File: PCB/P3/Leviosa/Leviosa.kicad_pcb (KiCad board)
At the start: 2 copper layers, 78.2 x 75.4 mm, 55 parts, among them J1 Barrel_Jack, J2 2.54mm 1x03 Spare, Q1 NCE0110K

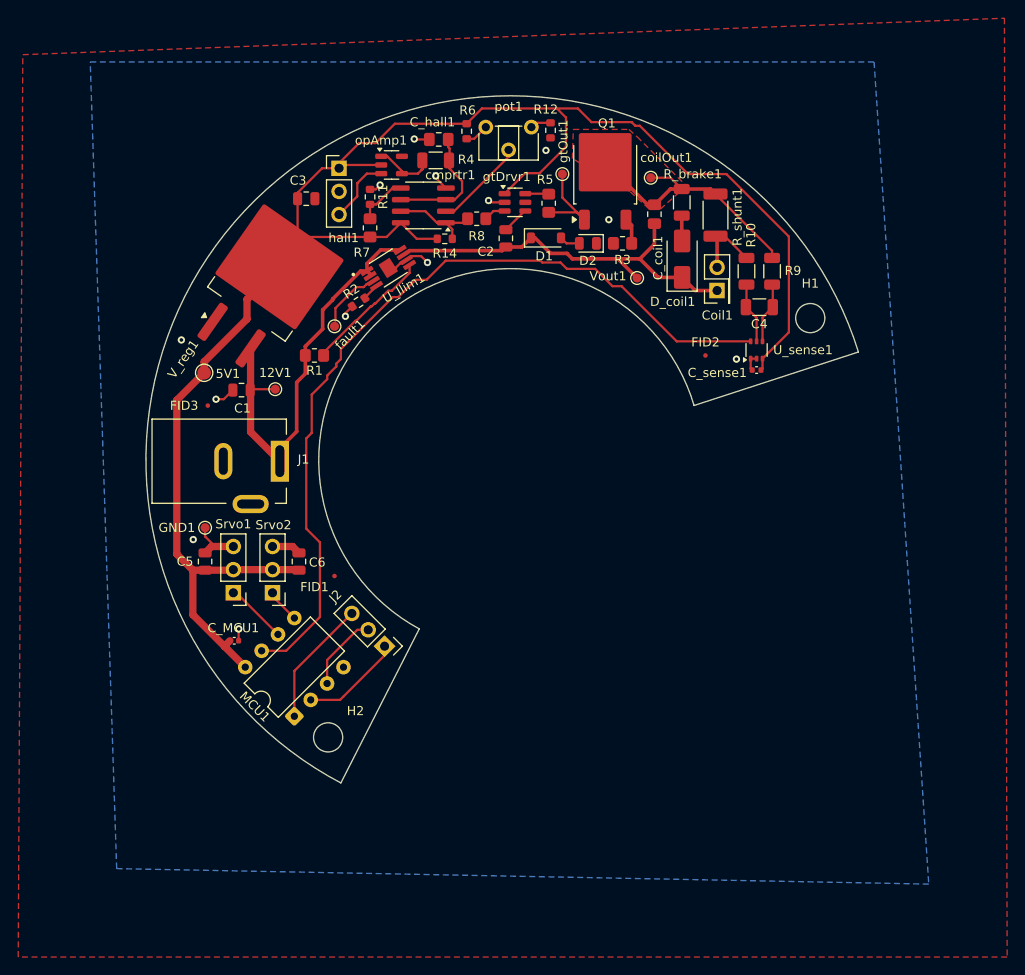
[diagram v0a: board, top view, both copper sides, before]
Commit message: Board revised
- Big change from the last so have a look over
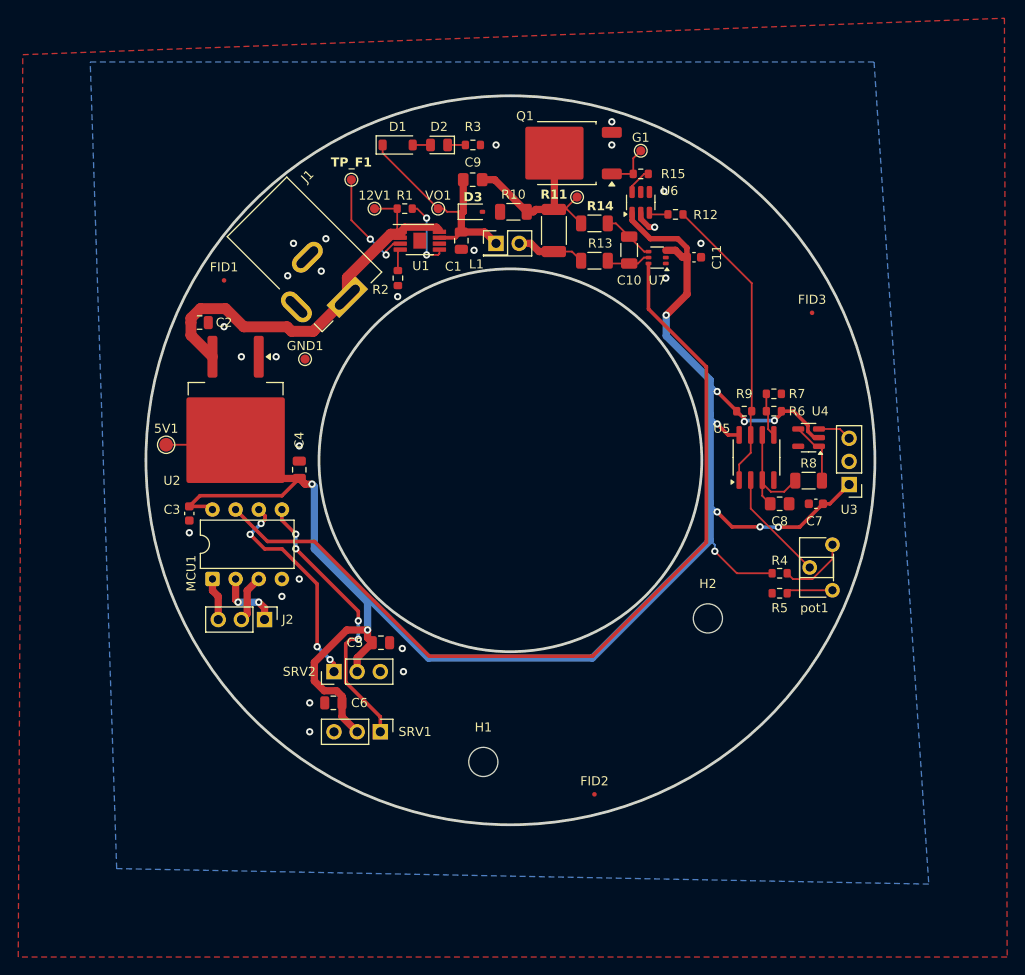
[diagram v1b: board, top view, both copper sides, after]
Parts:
- removed C_MCU1, C_sense1: 0.1µF, Capacitor_SMD:C_0402_1005Metric
- removed C_coil1: 20nF, Capacitor_SMD:C_0805_2012Metric_Pad1.18x1.45mm_HandSolder
- removed C_hall1: 4.7nF, Capacitor_SMD:C_0805_2012Metric_Pad1.18x1.45mm_HandSolder
- removed Coil1: 7.4mH, Connector_PinHeader_2.54mm:PinHeader_2x01_P2.54mm_Vertical
- removed D_coil1: SS34, Diode_SMD:D_SMA
- removed R_brake1: 8.2Ω, Resistor_SMD:R_1206_3216Metric
- removed R_shunt1: 50mΩ, Resistor_SMD:R_2010_5025Metric
- removed Srvo1, Srvo2: 2.54mm 1x03 Servo 1, Connector_PinHeader_2.54mm:PinHeader_1x03_P2.54mm_Vertical
- removed U_Ilim1: TPS1H200AQDGNRQ1, TPS1H200AQDGNRQ1:SOP65P490X110-9N
- removed U_sense1: INA199xxDCK (50V/V), Package_TO_SOT_SMD:SOT-363_SC-70-6
- removed V_reg1: MC7805BD2TR4G, Package_TO_SOT_SMD:TO-263-2
- removed Vout1: Vout, TestPoint:TestPoint_Pad_D1.0mm
- removed cmprtr1: LM393, Package_SO:SOIC-8_3.9x4.9mm_P1.27mm
- removed coilOut1: coil_out, TestPoint:TestPoint_Pad_D1.0mm
- removed fault1: Fault, TestPoint:TestPoint_Pad_D1.0mm
- removed gtDrvr1: MX27517, Package_TO_SOT_SMD:SOT-23-6
- removed gtOut1: set_point_trigger, TestPoint:TestPoint_Pad_D1.0mm
- removed hall1: SS495A, Connector_PinHeader_2.54mm:PinHeader_1x03_P2.54mm_Vertical
- removed opAmp1: MCP6001R, Package_TO_SOT_SMD:SOT-23-5
- added C10: 47μF, Capacitor_SMD:C_1206_3216Metric, F.Cu at (113.0, 76.9)
- added C11: 0.1µF, Capacitor_SMD:C_0603_1608Metric, F.Cu at (120.1, 77.7)
- added C7: 0.1uF, Capacitor_SMD:C_0603_1608Metric, F.Cu at (133.5, 104.8)
- added C8: 4.7nF, Capacitor_SMD:C_0805_2012Metric_Pad1.18x1.45mm_HandSolder, F.Cu at (129.5, 104.8)
- added C9: 20nF, Capacitor_SMD:C_0805_2012Metric_Pad1.18x1.45mm_HandSolder, F.Cu at (95.9, 69.2)
- added D3: SS34, Diode_SMD:D_SOD-323, F.Cu at (95.9, 72.7)
- added G1: set_point_trigger, TestPoint:TestPoint_Pad_D1.0mm, F.Cu at (114.3, 66.0)
- added L1: 7.4mH, Connector_PinHeader_2.54mm:PinHeader_2x01_P2.54mm_Vertical, F.Cu at (98.4, 76.2)
- added R13: 8.2Ω, Resistor_SMD:R_1206_3216Metric, F.Cu at (109.2, 78.1)
- added R15: 0Ω, Resistor_SMD:R_0603_1608Metric, F.Cu at (114.3, 68.6)
- added SRV1: 2.54mm 1x03 Servo 1, Connector_PinHeader_2.54mm:PinHeader_1x03_P2.54mm_Vertical, F.Cu at (85.7, 129.8)
- added SRV2: 2.54mm 1x03 Servo 1, Connector_PinHeader_2.54mm:PinHeader_1x03_P2.54mm_Vertical, F.Cu at (80.6, 123.2)
- added TP_COIL1: Coil Output, TestPoint:TestPoint_Pad_D1.0mm, F.Cu at (107.3, 71.1)
- added TP_F1: Fault, TestPoint:TestPoint_Pad_D1.0mm, F.Cu at (82.5, 69.2)
- added U1: TPS1H200AQDGNRQ1, TPS1H200AQDGNRQ1:SOP65P490X110-9N, F.Cu at (90.1, 75.9)
- added U2: MC7805BD2TR4G, Package_TO_SOT_SMD:TO-263-2, F.Cu at (69.8, 96.3)
- added U3: SS495A, Connector_PinHeader_2.54mm:PinHeader_1x03_P2.54mm_Vertical, F.Cu at (137.2, 102.7)
- added U4: MCP6001R, Package_TO_SOT_SMD:SOT-23-5, F.Cu at (132.7, 97.5)
- added U5: LM393, Package_SO:SOIC-8_3.9x4.9mm_P1.27mm, F.Cu at (127.0, 99.7)
- added U6: MX27517, Package_TO_SOT_SMD:SOT-23-6, F.Cu at (114.3, 71.7)
- added U7: INA199xxDCK (50V/V), Package_TO_SOT_SMD:SOT-363_SC-70-6, F.Cu at (116.1, 77.8)
- added VO1: Vout, TestPoint:TestPoint_Pad_D1.0mm, F.Cu at (92.1, 72.4)
- C1: value 0.33µF -> 22µF
- C2: value 22µF -> 0.33µF
- C3: value 0.33µF -> 0.1µF; footprint Capacitor_SMD:C_0805_2012Metric -> Capacitor_SMD:C_0603_1608Metric
- C4: value 47μF -> 0.33µF; footprint Capacitor_SMD:C_1206_3216Metric -> Capacitor_SMD:C_0805_2012Metric
- R1, R3: footprint Resistor_SMD:R_0805_2012Metric_Pad1.20x1.40mm_HandSolder -> Resistor_SMD:R_0603_1608Metric
- R11: value 68kΩ -> 50mΩ; footprint Resistor_SMD:R_0603_1608Metric -> Resistor_SMD:R_2010_5025Metric
- R12: value 3.9kΩ -> 0Ω
- R14: value 3.9kΩ -> 8.2Ω; footprint Resistor_SMD:R_0603_1608Metric -> Resistor_SMD:R_1206_3216Metric
- R4: value 8.2Ω -> 51kΩ; footprint Resistor_SMD:R_1206_3216Metric -> Resistor_SMD:R_0603_1608Metric
- R5: value 0Ω -> 3.9kΩ; footprint Resistor_SMD:R_0805_2012Metric_Pad1.20x1.40mm_HandSolder -> Resistor_SMD:R_0603_1608Metric
- R6: value 51kΩ -> 100kΩ
- R7: value 100kΩ -> 68kΩ; footprint Resistor_SMD:R_0805_2012Metric_Pad1.20x1.40mm_HandSolder -> Resistor_SMD:R_0603_1608Metric
- R8: value 0Ω -> 8.2Ω; footprint Resistor_SMD:R_0805_2012Metric_Pad1.20x1.40mm_HandSolder -> Resistor_SMD:R_1206_3216Metric
- R9: value 8.2Ω -> 3.9kΩ; footprint Resistor_SMD:R_1206_3216Metric -> Resistor_SMD:R_0603_1608Metric
- moved FID3 67.1 mm to (133.1, 83.8)
- moved pot1 60.6 mm to (135.3, 114.3), turned to 180 degrees
- moved H1 60.5 mm to (97.0, 133.1)
- moved R4 59.0 mm to (129.5, 112.4), turned to 180 degrees
- moved C4 53.5 mm to (76.8, 101.0), turned to 90 degrees
- moved R5 49.7 mm to (129.5, 114.6), turned to 0 degrees
- moved FID2 49.7 mm to (109.2, 136.7)
- moved R7 47.9 mm to (128.9, 92.7), turned to 180 degrees
- moved R8 46.4 mm to (132.7, 102.2), turned to 180 degrees
- moved R6 45.6 mm to (128.9, 94.6), turned to 0 degrees
- moved H2 43.7 mm to (121.7, 117.3)
- moved C3 36.8 mm to (64.8, 105.8), turned to -90 degrees
- moved C2 34.8 mm to (65.9, 84.9), turned to 0 degrees
- moved FID1 34.6 mm to (68.6, 80.3)
- moved C1 29.2 mm to (94.6, 75.9), turned to -90 degrees
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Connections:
- 5V1 pad 1: /5V -> +5V
- C1 pad 1: +12V -> +12V_SF
- C2 pad 1: /V_out -> +12V
- C3 pad 1: /5V -> +5V
- C4 pad 1: Net-(U_sense1-+) -> +5V
- C4 pad 2: Net-(U_sense1--) -> GND
- C5 pad 1: /5V -> +5V
- C6 pad 1: /5V -> +5V
- D1 pad 1: /V_out -> +12V_SF
- MCU1 pad 5: /servo2_control -> /SVR2_CTRL
- MCU1 pad 6: /servo1_control -> /SVR1_CTRL
- MCU1 pad 7: /current_sense -> /CURT_SN
- MCU1 pad 8: /5V -> +5V
- Q1 pad 1: /gate_driver_out -> /GT_DRV
- Q1 pad 2: /coil_output -> /COIL_OUT
- R10 pad 2: Net-(U_sense1--) -> /COIL_OUT
- R11 pad 1: GND -> Net-(L1-Pad2)
- R11 pad 2: /no_magnet_point -> /COIL_OUT
- R12 pad 1: GND -> /COMP_OUT
- R12 pad 2: Net-(R12-Pad2) -> Net-(U6-IN+)
- R14 pad 1: /comparator_out -> /COIL_OUT
- R14 pad 2: /5V -> Net-(U7-+)
- R4 pad 1: /instrumental_out -> Net-(R4-Pad1)
- R4 pad 2: Net-(cmprtr1A-+) -> +5V
- R5 pad 1: Net-(gtDrvr1-OUT) -> GND
- R5 pad 2: /gate_driver_out -> Net-(R5-Pad2)
- R6 pad 1: Net-(R6-Pad1) -> /NO_MGNT_PT
- R6 pad 2: /5V -> +5V
- R7 pad 1: /no_magnet_point -> GND
- R7 pad 2: /5V -> /NO_MGNT_PT
- R8 pad 1: /comparator_out -> /INST_OUT
- R9 pad 1: /coil_output -> /COMP_OUT
- R9 pad 2: Net-(U_sense1-+) -> +5V
- pot1 pad 1: Net-(R12-Pad2) -> Net-(R5-Pad2)
- pot1 pad 2: /set_point -> /SET_PT
- pot1 pad 3: Net-(R6-Pad1) -> Net-(R4-Pad1)
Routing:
- net +5V: track 0.00 -> 215.3 mm, vias 0 -> 11
- net /5V: track 193.7 -> 0.00 mm
- net /CURT_SN: track 0.00 -> 96.7 mm
- net /current_sense: track 92.2 -> 0.00 mm
- net /V_out: track 44.3 -> 0.00 mm
- net /COMP_OUT: track 0.00 -> 32.8 mm
- net /SVR2_CTRL: track 0.00 -> 30.5 mm, vias 0 -> 4
- net GND: track 32.8 -> 2.57 mm, vias 13 -> 24
- net /coil_output: track 28.3 -> 0.00 mm
- net +12V_SF: track 0.00 -> 25.2 mm
- net /SVR1_CTRL: track 0.00 -> 23.7 mm, vias 0 -> 4
- net /COIL_OUT: track 0.00 -> 22.4 mm
- net Net-(cmprtr1A-+): track 13.5 -> 0.00 mm
- net /SET_PT: track 0.00 -> 12.3 mm
- net Net-(U1-~{FAULT}): track 0.00 -> 12.1 mm, vias 0 -> 2
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- removed copper zone on F.Cu, net /coil_output
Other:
- board size 78.2 x 75.4 mm -> 80 x 80 mm
